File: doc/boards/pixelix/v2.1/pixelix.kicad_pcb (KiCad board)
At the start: 2 copper layers, 88.9 x 88.9 mm, 3 parts, among them J1 , U1 ESP32-WROOM, U4 CP2102N-Axx-xQFN28

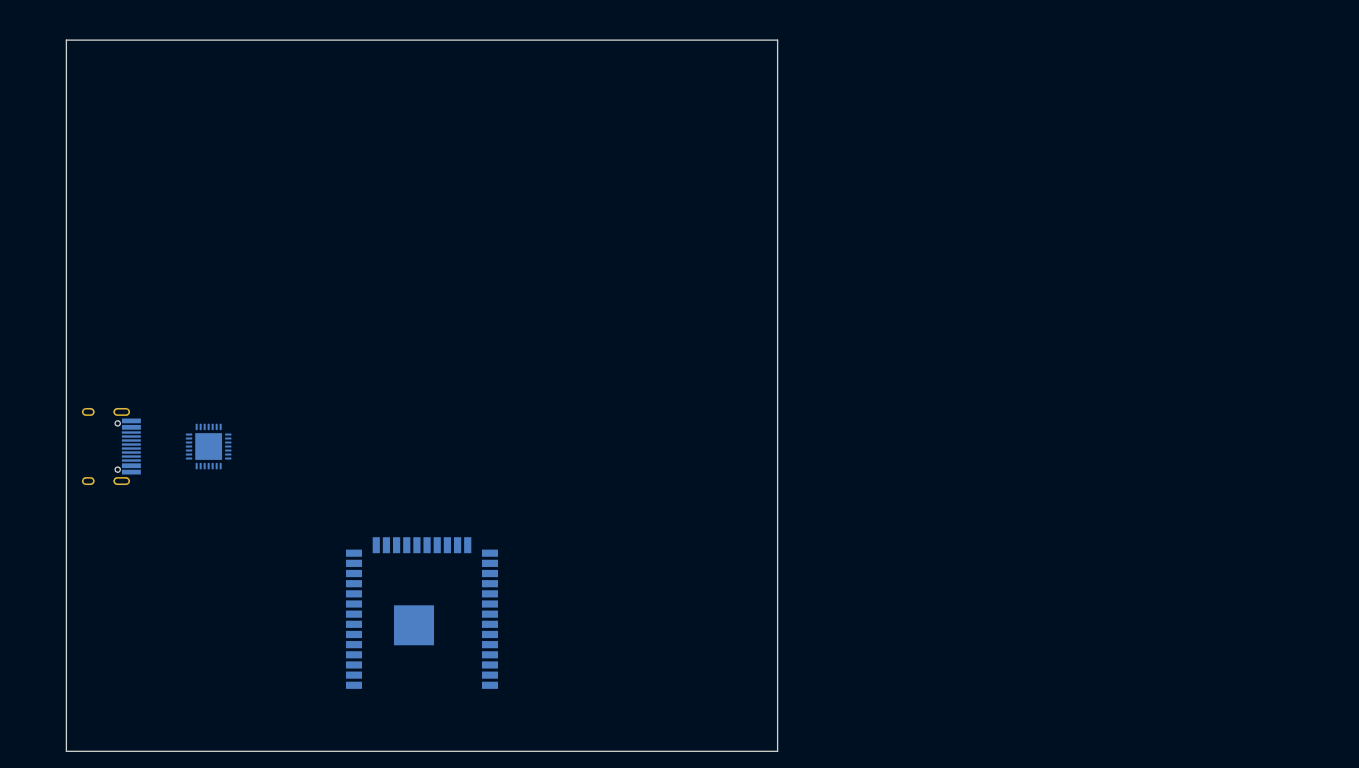
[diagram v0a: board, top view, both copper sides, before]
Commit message: Update file kicad
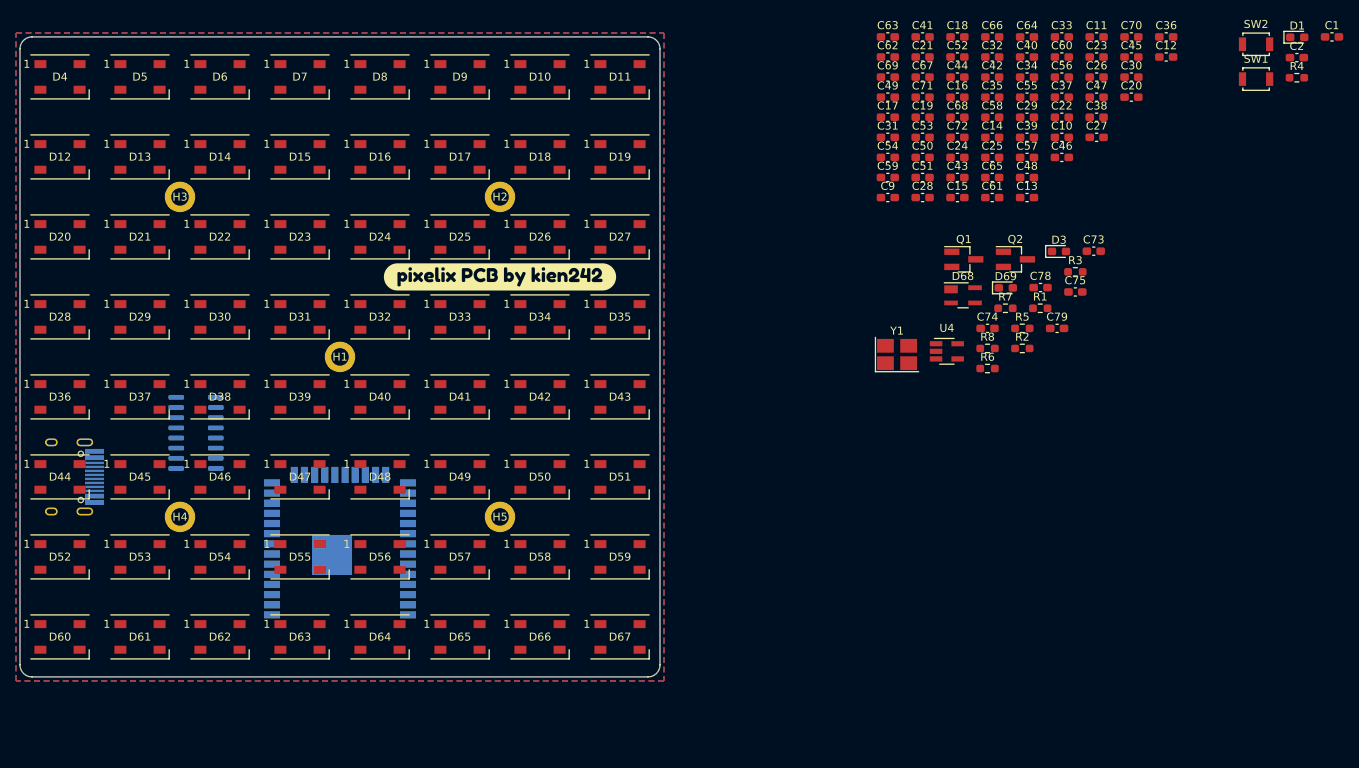
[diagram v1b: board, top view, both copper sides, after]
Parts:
- added C1: 1nf, Capacitor_SMD:C_0603_1608Metric_Pad1.08x0.95mm_HandSolder, F.Cu at (209.0, 25.0)
- added C10: 104, Capacitor_SMD:C_0603_1608Metric_Pad1.08x0.95mm_HandSolder, F.Cu at (175.2, 37.5)
- added C11: 104, Capacitor_SMD:C_0603_1608Metric_Pad1.08x0.95mm_HandSolder, F.Cu at (179.6, 25.0)
- added C12: 104, Capacitor_SMD:C_0603_1608Metric_Pad1.08x0.95mm_HandSolder, F.Cu at (188.3, 27.5)
- added C13: 104, Capacitor_SMD:C_0603_1608Metric_Pad1.08x0.95mm_HandSolder, F.Cu at (170.9, 45.1)
- added C14: 104, Capacitor_SMD:C_0603_1608Metric_Pad1.08x0.95mm_HandSolder, F.Cu at (166.5, 37.5)
- added C15: 104, Capacitor_SMD:C_0603_1608Metric_Pad1.08x0.95mm_HandSolder, F.Cu at (162.2, 45.1)
- added C16: 104, Capacitor_SMD:C_0603_1608Metric_Pad1.08x0.95mm_HandSolder, F.Cu at (162.2, 32.5)
- added C17: 104, Capacitor_SMD:C_0603_1608Metric_Pad1.08x0.95mm_HandSolder, F.Cu at (153.5, 35.0)
- added C18: 104, Capacitor_SMD:C_0603_1608Metric_Pad1.08x0.95mm_HandSolder, F.Cu at (162.2, 25.0)
- added C19: 104, Capacitor_SMD:C_0603_1608Metric_Pad1.08x0.95mm_HandSolder, F.Cu at (157.8, 35.0)
- added C2: 1nf, Capacitor_SMD:C_0603_1608Metric_Pad1.08x0.95mm_HandSolder, F.Cu at (204.6, 27.6)
- added C20: 104, Capacitor_SMD:C_0603_1608Metric_Pad1.08x0.95mm_HandSolder, F.Cu at (183.9, 32.5)
- added C21: 104, Capacitor_SMD:C_0603_1608Metric_Pad1.08x0.95mm_HandSolder, F.Cu at (157.8, 27.5)
- added C22: 104, Capacitor_SMD:C_0603_1608Metric_Pad1.08x0.95mm_HandSolder, F.Cu at (175.2, 35.0)
- added C23: 104, Capacitor_SMD:C_0603_1608Metric_Pad1.08x0.95mm_HandSolder, F.Cu at (179.6, 27.5)
- added C24: 104, Capacitor_SMD:C_0603_1608Metric_Pad1.08x0.95mm_HandSolder, F.Cu at (162.2, 40.1)
- added C25: 104, Capacitor_SMD:C_0603_1608Metric_Pad1.08x0.95mm_HandSolder, F.Cu at (166.5, 40.1)
- added C26: 104, Capacitor_SMD:C_0603_1608Metric_Pad1.08x0.95mm_HandSolder, F.Cu at (179.6, 30.0)
- added C27: 104, Capacitor_SMD:C_0603_1608Metric_Pad1.08x0.95mm_HandSolder, F.Cu at (179.6, 37.5)
- added C28: 104, Capacitor_SMD:C_0603_1608Metric_Pad1.08x0.95mm_HandSolder, F.Cu at (157.8, 45.1)
- added C29: 104, Capacitor_SMD:C_0603_1608Metric_Pad1.08x0.95mm_HandSolder, F.Cu at (170.9, 35.0)
- added C30: 104, Capacitor_SMD:C_0603_1608Metric_Pad1.08x0.95mm_HandSolder, F.Cu at (183.9, 30.0)
- added C31: 104, Capacitor_SMD:C_0603_1608Metric_Pad1.08x0.95mm_HandSolder, F.Cu at (153.5, 37.5)
- added C32: 104, Capacitor_SMD:C_0603_1608Metric_Pad1.08x0.95mm_HandSolder, F.Cu at (166.5, 27.5)
- added C33: 104, Capacitor_SMD:C_0603_1608Metric_Pad1.08x0.95mm_HandSolder, F.Cu at (175.2, 25.0)
- added C34: 104, Capacitor_SMD:C_0603_1608Metric_Pad1.08x0.95mm_HandSolder, F.Cu at (170.9, 30.0)
- added C35: 104, Capacitor_SMD:C_0603_1608Metric_Pad1.08x0.95mm_HandSolder, F.Cu at (166.5, 32.5)
- added C36: 104, Capacitor_SMD:C_0603_1608Metric_Pad1.08x0.95mm_HandSolder, F.Cu at (188.3, 25.0)
- added C37: 104, Capacitor_SMD:C_0603_1608Metric_Pad1.08x0.95mm_HandSolder, F.Cu at (175.2, 32.5)
- added C38: 104, Capacitor_SMD:C_0603_1608Metric_Pad1.08x0.95mm_HandSolder, F.Cu at (179.6, 35.0)
- added C39: 104, Capacitor_SMD:C_0603_1608Metric_Pad1.08x0.95mm_HandSolder, F.Cu at (170.9, 37.5)
- added C40: 104, Capacitor_SMD:C_0603_1608Metric_Pad1.08x0.95mm_HandSolder, F.Cu at (170.9, 27.5)
- added C41: 104, Capacitor_SMD:C_0603_1608Metric_Pad1.08x0.95mm_HandSolder, F.Cu at (157.8, 25.0)
- added C42: 104, Capacitor_SMD:C_0603_1608Metric_Pad1.08x0.95mm_HandSolder, F.Cu at (166.5, 30.0)
- added C43: 104, Capacitor_SMD:C_0603_1608Metric_Pad1.08x0.95mm_HandSolder, F.Cu at (162.2, 42.6)
- added C44: 104, Capacitor_SMD:C_0603_1608Metric_Pad1.08x0.95mm_HandSolder, F.Cu at (162.2, 30.0)
- added C45: 104, Capacitor_SMD:C_0603_1608Metric_Pad1.08x0.95mm_HandSolder, F.Cu at (183.9, 27.5)
- added C46: 104, Capacitor_SMD:C_0603_1608Metric_Pad1.08x0.95mm_HandSolder, F.Cu at (175.2, 40.1)
- added C47: 104, Capacitor_SMD:C_0603_1608Metric_Pad1.08x0.95mm_HandSolder, F.Cu at (179.6, 32.5)
- added C48: 104, Capacitor_SMD:C_0603_1608Metric_Pad1.08x0.95mm_HandSolder, F.Cu at (170.9, 42.6)
- added C49: 104, Capacitor_SMD:C_0603_1608Metric_Pad1.08x0.95mm_HandSolder, F.Cu at (153.5, 32.5)
- added C50: 104, Capacitor_SMD:C_0603_1608Metric_Pad1.08x0.95mm_HandSolder, F.Cu at (157.8, 40.1)
- added C51: 104, Capacitor_SMD:C_0603_1608Metric_Pad1.08x0.95mm_HandSolder, F.Cu at (157.8, 42.6)
- added C52: 104, Capacitor_SMD:C_0603_1608Metric_Pad1.08x0.95mm_HandSolder, F.Cu at (162.2, 27.5)
- added C53: 104, Capacitor_SMD:C_0603_1608Metric_Pad1.08x0.95mm_HandSolder, F.Cu at (157.8, 37.5)
- added C54: 104, Capacitor_SMD:C_0603_1608Metric_Pad1.08x0.95mm_HandSolder, F.Cu at (153.5, 40.1)
- added C55: 104, Capacitor_SMD:C_0603_1608Metric_Pad1.08x0.95mm_HandSolder, F.Cu at (170.9, 32.5)
- added C56: 104, Capacitor_SMD:C_0603_1608Metric_Pad1.08x0.95mm_HandSolder, F.Cu at (175.2, 30.0)
- added C57: 104, Capacitor_SMD:C_0603_1608Metric_Pad1.08x0.95mm_HandSolder, F.Cu at (170.9, 40.1)
- added C58: 104, Capacitor_SMD:C_0603_1608Metric_Pad1.08x0.95mm_HandSolder, F.Cu at (166.5, 35.0)
- added C59: 104, Capacitor_SMD:C_0603_1608Metric_Pad1.08x0.95mm_HandSolder, F.Cu at (153.5, 42.6)
- added C60: 104, Capacitor_SMD:C_0603_1608Metric_Pad1.08x0.95mm_HandSolder, F.Cu at (175.2, 27.5)
- added C61: 104, Capacitor_SMD:C_0603_1608Metric_Pad1.08x0.95mm_HandSolder, F.Cu at (166.5, 45.1)
- added C62: 104, Capacitor_SMD:C_0603_1608Metric_Pad1.08x0.95mm_HandSolder, F.Cu at (153.5, 27.5)
- added C63: 104, Capacitor_SMD:C_0603_1608Metric_Pad1.08x0.95mm_HandSolder, F.Cu at (153.5, 25.0)
- added C64: 104, Capacitor_SMD:C_0603_1608Metric_Pad1.08x0.95mm_HandSolder, F.Cu at (170.9, 25.0)
- added C65: 104, Capacitor_SMD:C_0603_1608Metric_Pad1.08x0.95mm_HandSolder, F.Cu at (166.5, 42.6)
- added C66: 104, Capacitor_SMD:C_0603_1608Metric_Pad1.08x0.95mm_HandSolder, F.Cu at (166.5, 25.0)
- added C67: 104, Capacitor_SMD:C_0603_1608Metric_Pad1.08x0.95mm_HandSolder, F.Cu at (157.8, 30.0)
- added C68: 104, Capacitor_SMD:C_0603_1608Metric_Pad1.08x0.95mm_HandSolder, F.Cu at (162.2, 35.0)
- added C69: 104, Capacitor_SMD:C_0603_1608Metric_Pad1.08x0.95mm_HandSolder, F.Cu at (153.5, 30.0)
- added C70: 104, Capacitor_SMD:C_0603_1608Metric_Pad1.08x0.95mm_HandSolder, F.Cu at (183.9, 25.0)
- added C71: 104, Capacitor_SMD:C_0603_1608Metric_Pad1.08x0.95mm_HandSolder, F.Cu at (157.8, 32.5)
- added C72: 104, Capacitor_SMD:C_0603_1608Metric_Pad1.08x0.95mm_HandSolder, F.Cu at (162.2, 37.5)
- added C73: 10uF, Capacitor_SMD:C_0603_1608Metric_Pad1.08x0.95mm_HandSolder, F.Cu at (179.2, 51.8)
- added C74: 10uF, Capacitor_SMD:C_0603_1608Metric_Pad1.08x0.95mm_HandSolder, F.Cu at (165.9, 61.4)
- added C75: 100nF, Capacitor_SMD:C_0603_1608Metric_Pad1.08x0.95mm_HandSolder, F.Cu at (176.9, 56.9)
- added C78: 9pF, Capacitor_SMD:C_0603_1608Metric_Pad1.08x0.95mm_HandSolder, F.Cu at (172.6, 56.3)
- added C79: 9pF, Capacitor_SMD:C_0603_1608Metric_Pad1.08x0.95mm_HandSolder, F.Cu at (174.6, 61.4)
- added C9: 104, Capacitor_SMD:C_0603_1608Metric_Pad1.08x0.95mm_HandSolder, F.Cu at (153.5, 45.1)
- added D1: GREEN, LED_SMD:LED_0603_1608Metric_Pad1.05x0.95mm_HandSolder, F.Cu at (204.7, 25.0)
- added D10: , LED_SMD:LED_WS2812B_PLCC4_5.0x5.0mm_P3.2mm, F.Cu at (110.0, 30.0)
- added D11: , LED_SMD:LED_WS2812B_PLCC4_5.0x5.0mm_P3.2mm, F.Cu at (120.0, 30.0)
- added D12: , LED_SMD:LED_WS2812B_PLCC4_5.0x5.0mm_P3.2mm, F.Cu at (50.0, 40.0)
- added D13: , LED_SMD:LED_WS2812B_PLCC4_5.0x5.0mm_P3.2mm, F.Cu at (60.0, 40.0)
- added D14: , LED_SMD:LED_WS2812B_PLCC4_5.0x5.0mm_P3.2mm, F.Cu at (70.0, 40.0)
- added D15: , LED_SMD:LED_WS2812B_PLCC4_5.0x5.0mm_P3.2mm, F.Cu at (80.0, 40.0)
- added D16: , LED_SMD:LED_WS2812B_PLCC4_5.0x5.0mm_P3.2mm, F.Cu at (90.0, 40.0)
- added D17: , LED_SMD:LED_WS2812B_PLCC4_5.0x5.0mm_P3.2mm, F.Cu at (100.0, 40.0)
- added D18: , LED_SMD:LED_WS2812B_PLCC4_5.0x5.0mm_P3.2mm, F.Cu at (110.0, 40.0)
- added D19: , LED_SMD:LED_WS2812B_PLCC4_5.0x5.0mm_P3.2mm, F.Cu at (120.0, 40.0)
- added D20: , LED_SMD:LED_WS2812B_PLCC4_5.0x5.0mm_P3.2mm, F.Cu at (50.0, 50.0)
- added D21: , LED_SMD:LED_WS2812B_PLCC4_5.0x5.0mm_P3.2mm, F.Cu at (60.0, 50.0)
- added D22: , LED_SMD:LED_WS2812B_PLCC4_5.0x5.0mm_P3.2mm, F.Cu at (70.0, 50.0)
- added D23: , LED_SMD:LED_WS2812B_PLCC4_5.0x5.0mm_P3.2mm, F.Cu at (80.0, 50.0)
- added D24: , LED_SMD:LED_WS2812B_PLCC4_5.0x5.0mm_P3.2mm, F.Cu at (90.0, 50.0)
- added D25: , LED_SMD:LED_WS2812B_PLCC4_5.0x5.0mm_P3.2mm, F.Cu at (100.0, 50.0)
- added D26: , LED_SMD:LED_WS2812B_PLCC4_5.0x5.0mm_P3.2mm, F.Cu at (110.0, 50.0)
- added D27: , LED_SMD:LED_WS2812B_PLCC4_5.0x5.0mm_P3.2mm, F.Cu at (120.0, 50.0)
- added D28: , LED_SMD:LED_WS2812B_PLCC4_5.0x5.0mm_P3.2mm, F.Cu at (50.0, 60.0)
- added D29: , LED_SMD:LED_WS2812B_PLCC4_5.0x5.0mm_P3.2mm, F.Cu at (60.0, 60.0)
- added D3: RED, LED_SMD:LED_0603_1608Metric_Pad1.05x0.95mm_HandSolder, F.Cu at (174.9, 51.8)
- added D30: , LED_SMD:LED_WS2812B_PLCC4_5.0x5.0mm_P3.2mm, F.Cu at (70.0, 60.0)
- added D31: , LED_SMD:LED_WS2812B_PLCC4_5.0x5.0mm_P3.2mm, F.Cu at (80.0, 60.0)
- added D32: , LED_SMD:LED_WS2812B_PLCC4_5.0x5.0mm_P3.2mm, F.Cu at (90.0, 60.0)
- added D33: , LED_SMD:LED_WS2812B_PLCC4_5.0x5.0mm_P3.2mm, F.Cu at (100.0, 60.0)
- added D34: , LED_SMD:LED_WS2812B_PLCC4_5.0x5.0mm_P3.2mm, F.Cu at (110.0, 60.0)
- added D35: , LED_SMD:LED_WS2812B_PLCC4_5.0x5.0mm_P3.2mm, F.Cu at (120.0, 60.0)
- added D36: , LED_SMD:LED_WS2812B_PLCC4_5.0x5.0mm_P3.2mm, F.Cu at (50.0, 70.0)
- added D37: , LED_SMD:LED_WS2812B_PLCC4_5.0x5.0mm_P3.2mm, F.Cu at (60.0, 70.0)
- added D38: , LED_SMD:LED_WS2812B_PLCC4_5.0x5.0mm_P3.2mm, F.Cu at (70.0, 70.0)
- added D39: , LED_SMD:LED_WS2812B_PLCC4_5.0x5.0mm_P3.2mm, F.Cu at (80.0, 70.0)
- added D4: , LED_SMD:LED_WS2812B_PLCC4_5.0x5.0mm_P3.2mm, F.Cu at (50.0, 30.0)
- added D40: , LED_SMD:LED_WS2812B_PLCC4_5.0x5.0mm_P3.2mm, F.Cu at (90.0, 70.0)
- added D41: , LED_SMD:LED_WS2812B_PLCC4_5.0x5.0mm_P3.2mm, F.Cu at (100.0, 70.0)
- added D42: , LED_SMD:LED_WS2812B_PLCC4_5.0x5.0mm_P3.2mm, F.Cu at (110.0, 70.0)
- added D43: , LED_SMD:LED_WS2812B_PLCC4_5.0x5.0mm_P3.2mm, F.Cu at (120.0, 70.0)
- added D44: , LED_SMD:LED_WS2812B_PLCC4_5.0x5.0mm_P3.2mm, F.Cu at (50.0, 80.0)
- added D45: , LED_SMD:LED_WS2812B_PLCC4_5.0x5.0mm_P3.2mm, F.Cu at (60.0, 80.0)
- added D46: , LED_SMD:LED_WS2812B_PLCC4_5.0x5.0mm_P3.2mm, F.Cu at (70.0, 80.0)
- added D47: , LED_SMD:LED_WS2812B_PLCC4_5.0x5.0mm_P3.2mm, F.Cu at (80.0, 80.0)
- added D48: , LED_SMD:LED_WS2812B_PLCC4_5.0x5.0mm_P3.2mm, F.Cu at (90.0, 80.0)
- added D49: , LED_SMD:LED_WS2812B_PLCC4_5.0x5.0mm_P3.2mm, F.Cu at (100.0, 80.0)
- added D5: , LED_SMD:LED_WS2812B_PLCC4_5.0x5.0mm_P3.2mm, F.Cu at (60.0, 30.0)
- added D50: , LED_SMD:LED_WS2812B_PLCC4_5.0x5.0mm_P3.2mm, F.Cu at (110.0, 80.0)
- added D51: , LED_SMD:LED_WS2812B_PLCC4_5.0x5.0mm_P3.2mm, F.Cu at (120.0, 80.0)
- added D52: , LED_SMD:LED_WS2812B_PLCC4_5.0x5.0mm_P3.2mm, F.Cu at (50.0, 90.0)
- added D53: , LED_SMD:LED_WS2812B_PLCC4_5.0x5.0mm_P3.2mm, F.Cu at (60.0, 90.0)
- added D54: , LED_SMD:LED_WS2812B_PLCC4_5.0x5.0mm_P3.2mm, F.Cu at (70.0, 90.0)
- added D55: , LED_SMD:LED_WS2812B_PLCC4_5.0x5.0mm_P3.2mm, F.Cu at (80.0, 90.0)
- added D56: , LED_SMD:LED_WS2812B_PLCC4_5.0x5.0mm_P3.2mm, F.Cu at (90.0, 90.0)
- added D57: , LED_SMD:LED_WS2812B_PLCC4_5.0x5.0mm_P3.2mm, F.Cu at (100.0, 90.0)
- added D58: , LED_SMD:LED_WS2812B_PLCC4_5.0x5.0mm_P3.2mm, F.Cu at (110.0, 90.0)
- added D59: , LED_SMD:LED_WS2812B_PLCC4_5.0x5.0mm_P3.2mm, F.Cu at (120.0, 90.0)
- added D6: , LED_SMD:LED_WS2812B_PLCC4_5.0x5.0mm_P3.2mm, F.Cu at (70.0, 30.0)
- added D60: , LED_SMD:LED_WS2812B_PLCC4_5.0x5.0mm_P3.2mm, F.Cu at (50.0, 100.0)
- added D61: , LED_SMD:LED_WS2812B_PLCC4_5.0x5.0mm_P3.2mm, F.Cu at (60.0, 100.0)
- added D62: , LED_SMD:LED_WS2812B_PLCC4_5.0x5.0mm_P3.2mm, F.Cu at (70.0, 100.0)
- added D63: , LED_SMD:LED_WS2812B_PLCC4_5.0x5.0mm_P3.2mm, F.Cu at (80.0, 100.0)
- added D64: , LED_SMD:LED_WS2812B_PLCC4_5.0x5.0mm_P3.2mm, F.Cu at (90.0, 100.0)
- added D65: , LED_SMD:LED_WS2812B_PLCC4_5.0x5.0mm_P3.2mm, F.Cu at (100.0, 100.0)
- added D66: , LED_SMD:LED_WS2812B_PLCC4_5.0x5.0mm_P3.2mm, F.Cu at (110.0, 100.0)
- added D67: , LED_SMD:LED_WS2812B_PLCC4_5.0x5.0mm_P3.2mm, F.Cu at (120.0, 100.0)
- added D68: PRTR5V0U2X, Package_TO_SOT_SMD:SOT-143_Handsoldering, F.Cu at (162.9, 57.3)
- added D69: GREEN, LED_SMD:LED_0603_1608Metric_Pad1.05x0.95mm_HandSolder, F.Cu at (168.2, 56.4)
- added D7: , LED_SMD:LED_WS2812B_PLCC4_5.0x5.0mm_P3.2mm, F.Cu at (80.0, 30.0)
- added D8: , LED_SMD:LED_WS2812B_PLCC4_5.0x5.0mm_P3.2mm, F.Cu at (90.0, 30.0)
- added D9: , LED_SMD:LED_WS2812B_PLCC4_5.0x5.0mm_P3.2mm, F.Cu at (100.0, 30.0)
- added H1: M2, MountingHole:MountingHole_2.2mm_M2_DIN965_Pad, F.Cu at (85.0, 65.0)
- added H2: M2, MountingHole:MountingHole_2.2mm_M2_DIN965_Pad, F.Cu at (105.0, 45.0)
- added H3: M2, MountingHole:MountingHole_2.2mm_M2_DIN965_Pad, F.Cu at (65.0, 45.0)
- added H4: M2, MountingHole:MountingHole_2.2mm_M2_DIN965_Pad, F.Cu at (65.0, 85.0)
- added H5: M2, MountingHole:MountingHole_2.2mm_M2_DIN965_Pad, F.Cu at (105.0, 85.0)
- added Q1: MMBT3904, Package_TO_SOT_SMD:SOT-23_Handsoldering, F.Cu at (163.0, 52.8)
- added Q2: MMBT3904, Package_TO_SOT_SMD:SOT-23_Handsoldering, F.Cu at (169.4, 52.8)
- added R1: 10K, Resistor_SMD:R_0603_1608Metric_Pad0.98x0.95mm_HandSolder, F.Cu at (172.5, 58.9)
- added R2: 10K, Resistor_SMD:R_0603_1608Metric_Pad0.98x0.95mm_HandSolder, F.Cu at (170.3, 63.9)
- added R3: 10K, Resistor_SMD:R_0603_1608Metric_Pad0.98x0.95mm_HandSolder, F.Cu at (176.9, 54.4)
- added R4: 10K, Resistor_SMD:R_0603_1608Metric_Pad0.98x0.95mm_HandSolder, F.Cu at (204.6, 30.1)
- added R5: 100, Resistor_SMD:R_0603_1608Metric_Pad0.98x0.95mm_HandSolder, F.Cu at (170.3, 61.4)
- added R6: 100, Resistor_SMD:R_0603_1608Metric_Pad0.98x0.95mm_HandSolder, F.Cu at (165.9, 66.5)
- added R7: 1K, Resistor_SMD:R_0603_1608Metric_Pad0.98x0.95mm_HandSolder, F.Cu at (168.2, 58.9)
- added R8: 1K, Resistor_SMD:R_0603_1608Metric_Pad0.98x0.95mm_HandSolder, F.Cu at (165.9, 63.9)
- added SW1: SWITCH_SPST, Button_Switch_SMD:SW_SPST_B3U-1000P, F.Cu at (199.5, 30.3)
- added SW2: SWITCH_SPST, Button_Switch_SMD:SW_SPST_B3U-1000P, F.Cu at (199.5, 25.9)
- added U5: CH340G, Package_SO:SOIC-16_3.9x9.9mm_P1.27mm, B.Cu at (67.0, 74.5)
- added Y1: 32.768kHz, Crystal:Crystal_SMD_SeikoEpson_TSX3225-4Pin_3.2x2.5mm_HandSoldering, F.Cu at (154.6, 64.7)
- added kibuzzard-62F63F5E: G***, kibuzzard-62F63F5E, F.Cu at (105.0, 55.0)
- U4: value CP2102N-Axx-xQFN28 -> AP2127K-3.3; footprint Package_DFN_QFN:QFN-28-1EP_5x5mm_P0.5mm_EP3.35x3.35mm -> Package_TO_SOT_SMD:SOT-23-5_HandSoldering; moved to F.Cu
- moved U4 93.0 mm to (160.9, 64.3)
- moved U1 13.5 mm to (85.0, 89.0)
- moved J1 5.97 mm to (50.0, 80.0)
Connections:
- U4 pad 1: unconnected-(U4-~{DCD}) -> +5V
- U4 pad 2: unconnected-(U4-~{RI}/CLK) -> GND
- U4 pad 3: GND -> +5V
- U4 pad 4: D+ -> unconnected-(U4-NC)
- U4 pad 5: D- -> +3V3
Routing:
- added copper zone on B.Cu, net GND
- added copper zone on F.Cu, net GND
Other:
- board size 88.9 x 88.9 mm -> 80 x 80 mm
